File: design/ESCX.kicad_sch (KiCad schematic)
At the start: 18 parts, among them J1 HALL_ENC, J4 SWD, J5 USB_OTG, SW1 SENSOR_VOLTAGE

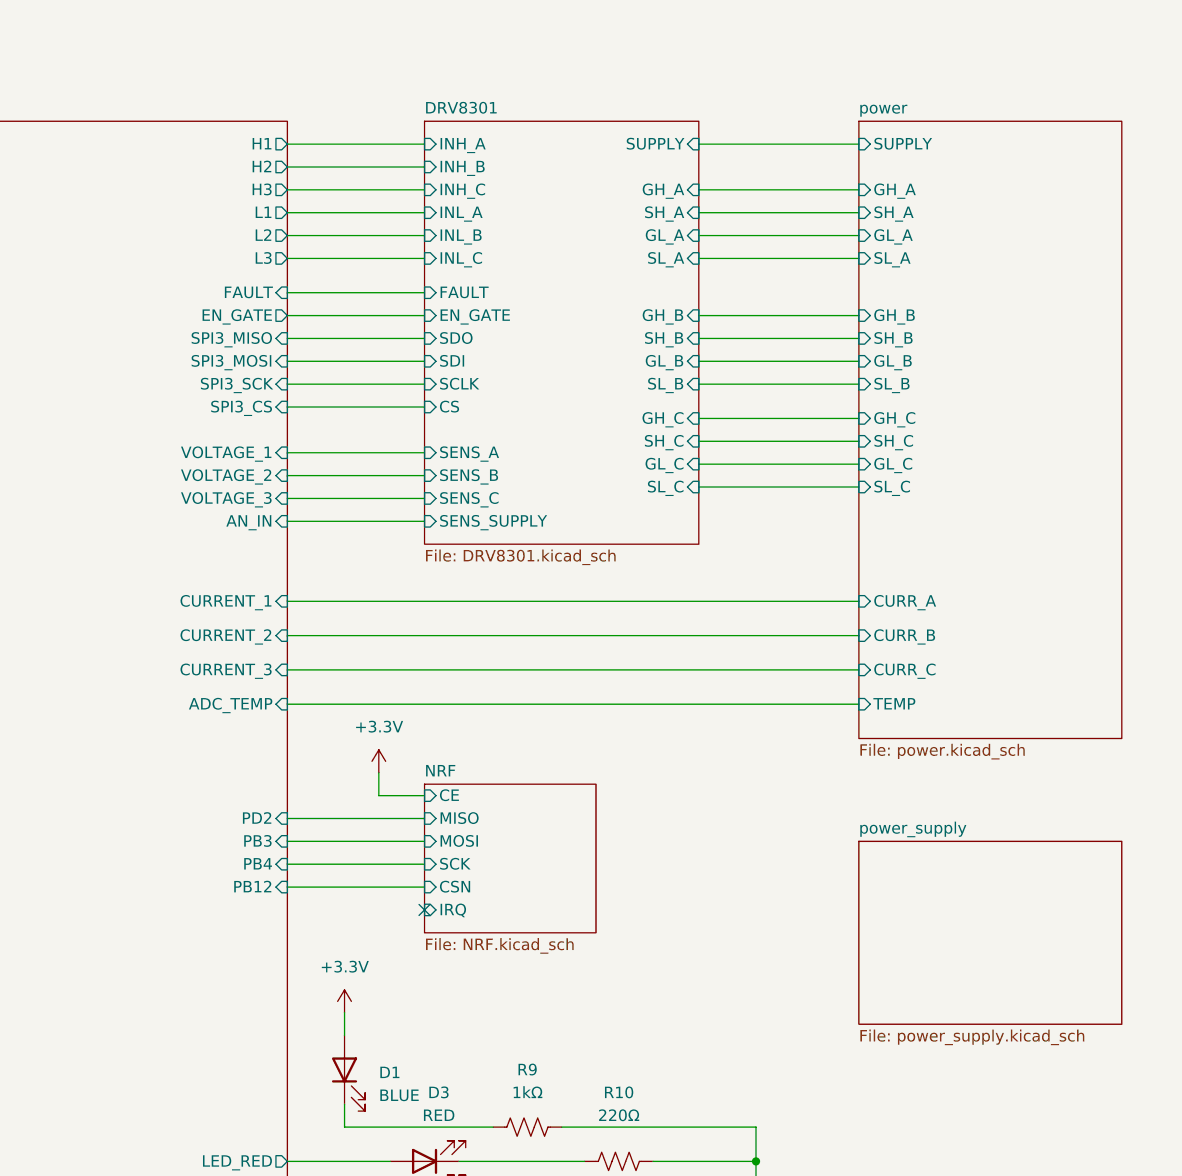
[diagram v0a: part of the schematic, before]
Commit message: Commit antes del merge
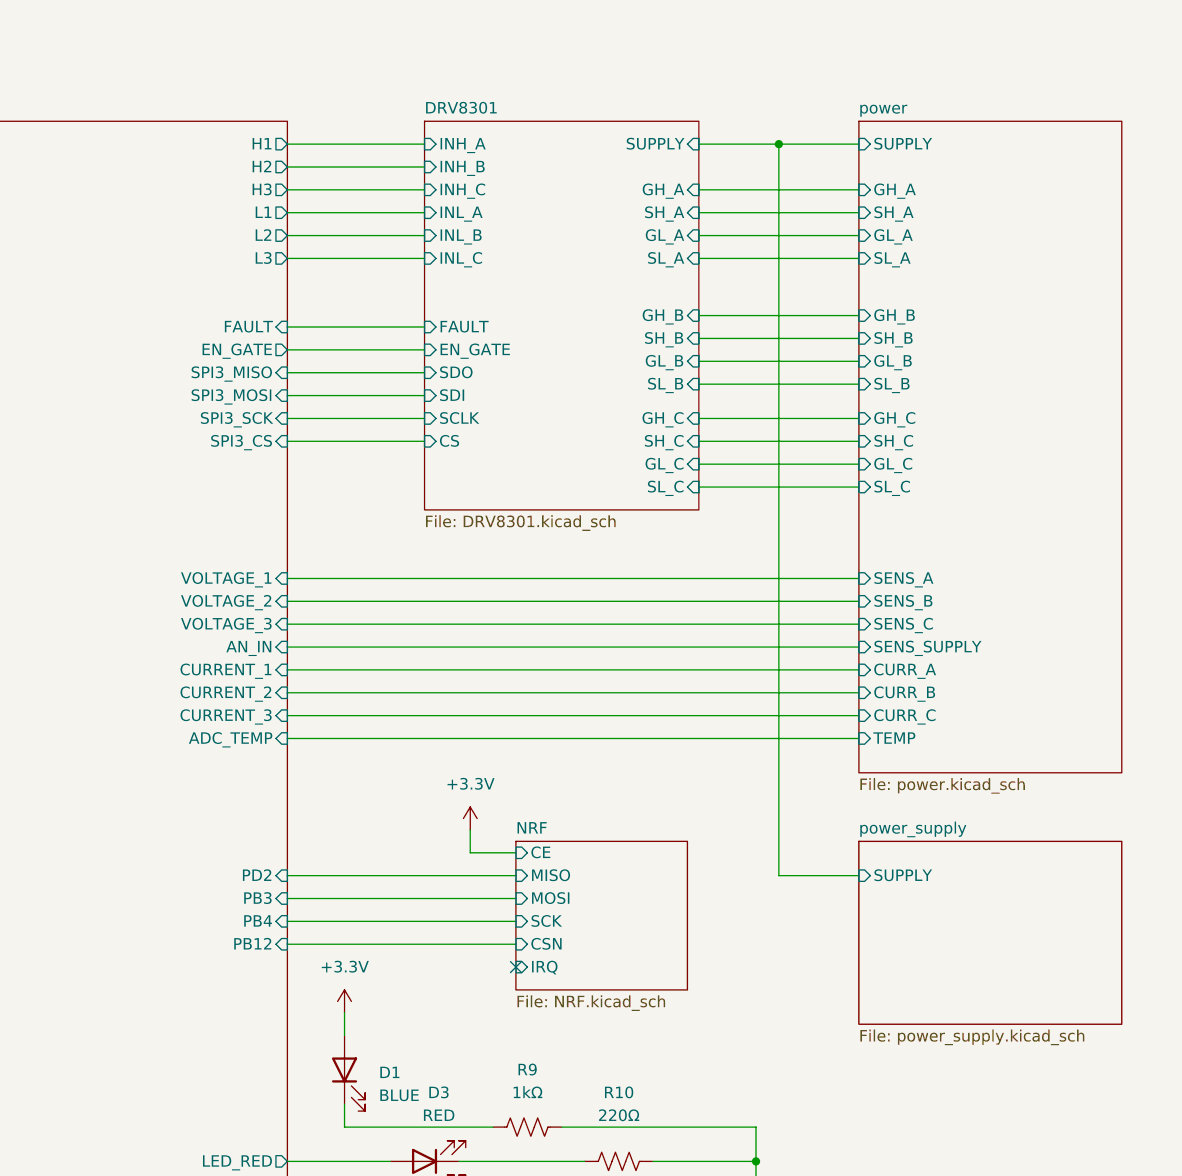
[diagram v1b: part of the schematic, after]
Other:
- sheet DRV8301 ports: added none; removed SENS_A, SENS_B, SENS_C, SENS_SUPPLY
- sheet power ports: added SENS_A, SENS_B, SENS_C, SENS_SUPPLY; removed none
- sheet power_supply ports: added SUPPLY; removed none
